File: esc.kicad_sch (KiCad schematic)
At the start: 10 parts, among them J1 Conn_01x02, J2 Conn_01x05, J3 Conn_01x03, U1 AP63205WU

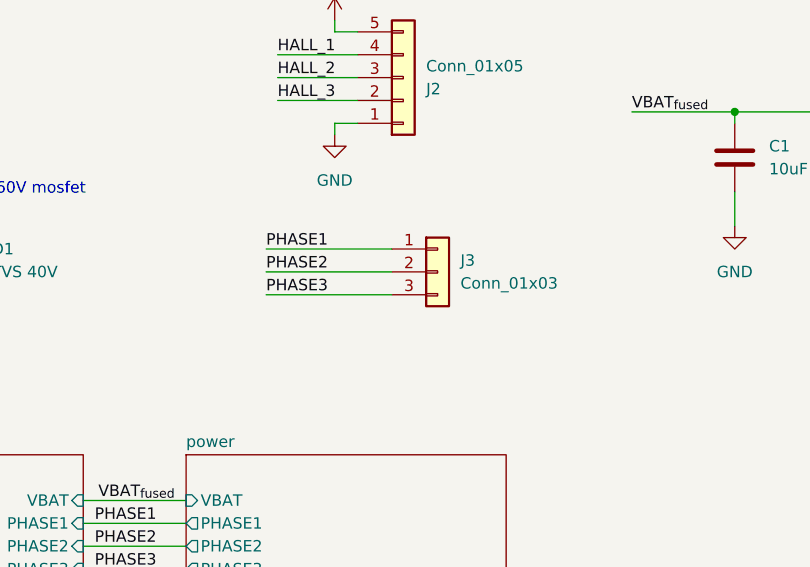
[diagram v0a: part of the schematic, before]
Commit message: added wire step
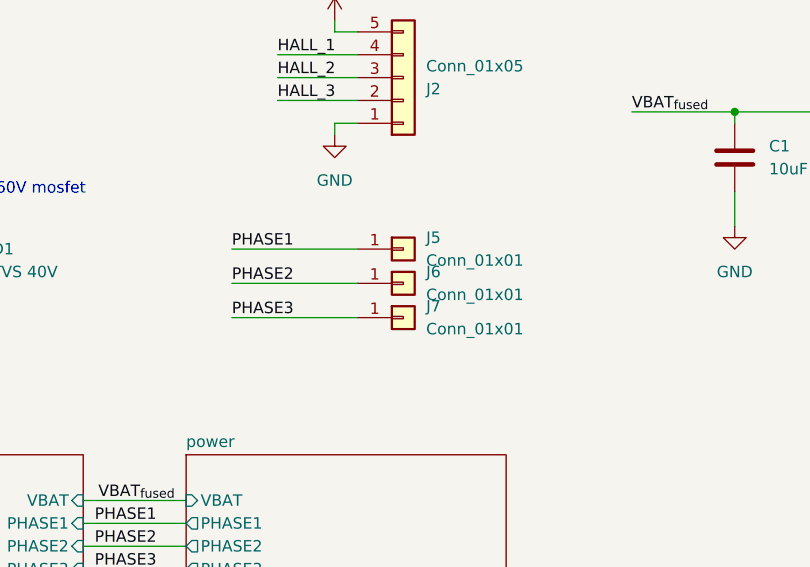
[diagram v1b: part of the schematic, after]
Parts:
- removed J3: Conn_01x03, symbol Connector_Generic:Conn_01x03
- added J5, J6, J7: Conn_01x01, MountingHole:MountingHole_3mm_Pad_Via, symbol Connector_Generic:Conn_01x01
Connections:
- net PHASE1: now also J5.1 (Pin_1)
- net PHASE2: now also J6.1 (Pin_1)
- net PHASE3: now also J7.1 (Pin_1)
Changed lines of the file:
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@@
 	(wire
 		(pts
-			(xy 222.25 96.52) (xy 236.22 96.52)
+			(xy 218.44 96.52) (xy 232.41 96.52)
 		)
 		(stroke
@@
 	(wire
 		(pts
-			(xy 222.25 101.6) (xy 236.22 101.6)
+			(xy 218.44 104.14) (xy 232.41 104.14)
 		)
 		(stroke
@@
 	(wire
 		(pts
-			(xy 222.25 99.06) (xy 236.22 99.06)
+			(xy 218.44 100.33) (xy 232.41 100.33)
 		)
 		(stroke
@@
 	)
 	(label "PHASE2"
-		(at 222.25 99.06 0)
+		(at 218.44 100.33 0)
 		(effects
 			(font
@@
 	)
 	(label "PHASE3"
-		(at 222.25 101.6 0)
+		(at 218.44 104.14 0)
 		(effects
 			(font
@@
 	)
 	(label "PHASE1"
-		(at 222.25 96.52 0)
+		(at 218.44 96.52 0)
 		(effects
 			(font
@@
 	)
 	(symbol
+		(lib_id "Connector_Generic:Conn_01x01")
+		(at 237.49 104.14 0)
+		(unit 1)
+		(body_style 1)
+		(exclude_from_sim no)
+		(in_bom yes)
+		(on_board yes)
+		(in_pos_files yes)
+		(dnp no)
+		(fields_autoplaced yes)
+		(property "Reference" "J7"
+			(at 240.03 102.8699 0)
+			(show_name no)
+			(do_not_autoplace no)
+			(effects
+				(font
+					(size 1.27 1.27)
+				)
+				(justify left)
+			)
+		)
+		(property "Value" "Conn_01x01"
+			(at 240.03 105.4099 0)
+			(show_name no)
+			(do_not_autoplace no)
+			(effects
+				(font
+					(size 1.27 1.27)
+				)
+				(justify left)
+			)
+		)
+		(property "Footprint" "MountingHole:MountingHole_3mm_Pad_Via"
+			(at 237.49 104.14 0)
+			(hide yes)
+			(show_name no)
+			(do_not_autoplace no)
+			(effects
+				(font
+					(size 1.27 1.27)
+				)
+			)
+		)
+		(property "Datasheet" ""
+			(at 237.49 104.14 0)
+			(hide yes)
+			(show_name no)
+			(do_not_autoplace no)
+			(effects
+				(font
+					(size 1.27 1.27)
+				)
+			)
+		)
+		(property "Description" "Generic connector, single row, 01x01, script generated (kicad-library-utils/schlib/autogen/connector/)"
+			(at 237.49 104.14 0)
+			(hide yes)
+			(show_name no)
+			(do_not_autoplace no)
+			(effects
+				(font
+					(size 1.27 1.27)
+				)
+			)
+		)
+		(pin "1"
+		)
+		(instances
+			(project "esc"
+				(path "/3007d2b9-1a69-4117-bc7c-a9e99ed2a97d"
+					(reference "J7")
+					(unit 1)
+				)
+			)
+		)
+	)
+	(symbol
+		(lib_id "Connector_Generic:Conn_01x01")
+		(at 237.49 100.33 0)
+		(unit 1)
+		(body_style 1)
+		(exclude_from_sim no)
+		(in_bom yes)
+		(on_board yes)
+		(in_pos_files yes)
+		(dnp no)
+		(fields_autoplaced yes)
+		(property "Reference" "J6"
+			(at 240.03 99.0599 0)
+			(show_name no)
+			(do_not_autoplace no)
+			(effects
+				(font
+					(size 1.27 1.27)
+				)
+				(justify left)
+			)
+		)
+		(property "Value" "Conn_01x01"
+			(at 240.03 101.5999 0)
+			(show_name no)
+			(do_not_autoplace no)
+			(effects
+				(font
+					(size 1.27 1.27)
+				)
+				(justify left)
+			)
+		)
+		(property "Footprint" "MountingHole:MountingHole_3mm_Pad_Via"
+			(at 237.49 100.33 0)
+			(hide yes)
+			(show_name no)
+			(do_not_autoplace no)
+			(effects
+				(font
+					(size 1.27 1.27)
+				)
+			)
+		)
+		(property "Datasheet" ""
+			(at 237.49 100.33 0)
+			(hide yes)
+			(show_name no)
+			(do_not_autoplace no)
+			(effects
+				(font
+					(size 1.27 1.27)
+				)
+			)
+		)
+		(property "Description" "Generic connector, single row, 01x01, script generated (kicad-library-utils/schlib/autogen/connector/)"
+			(at 237.49 100.33 0)
+			(hide yes)
+			(show_name no)
+			(do_not_autoplace no)
+			(effects
+				(font
+					(size 1.27 1.27)
+				)
+			)
+		)
+		(pin "1"
+		)
+		(instances
+			(project "esc"
+				(path "/3007d2b9-1a69-4117-bc7c-a9e99ed2a97d"
+					(reference "J6")
+					(unit 1)
+				)
+			)
+		)
+	)
+	(symbol
 		(lib_id "Device:C")
 		(at 318.77 83.82 90)
@@
 	)
 	(symbol
-		(lib_id "Connector_Generic:Conn_01x03")
-		(at 241.3 99.06 0)
+		(lib_id "Connector_Generic:Conn_01x01")
+		(at 237.49 96.52 0)
 		(unit 1)
 		(body_style 1)
@@
 		(dnp no)
 		(fields_autoplaced yes)
-		(property "Reference" "J3"
-			(at 243.84 97.7899 0)
+		(property "Reference" "J5"
+			(at 240.03 95.2499 0)
 			(show_name no)
 			(do_not_autoplace no)
@@
 			)
 		)
-		(property "Value" "Conn_01x03"
-			(at 243.84 100.3299 0)
+		(property "Value" "Conn_01x01"
+			(at 240.03 97.7899 0)
 			(show_name no)
 			(do_not_autoplace no)
@@
 			)
 		)
-		(property "Footprint" ""
-			(at 241.3 99.06 0)
+		(property "Footprint" "MountingHole:MountingHole_3mm_Pad_Via"
+			(at 237.49 96.52 0)
 			(hide yes)
 			(show_name no)
@@
 		)
 		(property "Datasheet" ""
-			(at 241.3 99.06 0)
-			(hide yes)
-			(show_name no)
-			(do_not_autoplace no)
-			(effects
-				(font
-					(size 1.27 1.27)
-				)
-			)
-		)
-		(property "Description" "Generic connector, single row, 01x03, script generated (kicad-library-utils/schlib/autogen/connector/)"
-			(at 241.3 99.06 0)
-			(hide yes)
-			(show_name no)
-			(do_not_autoplace no)
-			(effects
-				(font
-					(size 1.27 1.27)
-				)
-			)
-		)
-		(property "Sim.Device" ""
-			(at 241.3 99.06 0)
-			(hide yes)
-			(show_name no)
-			(do_not_autoplace no)
-			(effects
-				(font
-					(size 1.27 1.27)
-				)
-			)
-		)
-		(property "Sim.Type" ""
-			(at 241.3 99.06 0)
-			(hide yes)
-			(show_name no)
-			(do_not_autoplace no)
-			(effects
-				(font
-					(size 1.27 1.27)
-				)
-			)
-		)
-		(pin "3"
-		)
-		(pin "2"
+			(at 237.49 96.52 0)
+			(hide yes)
+			(show_name no)
+			(do_not_autoplace no)
+			(effects
+				(font
+					(size 1.27 1.27)
+				)
+			)
+		)
+		(property "Description" "Generic connector, single row, 01x01, script generated (kicad-library-utils/schlib/autogen/connector/)"
+			(at 237.49 96.52 0)
+			(hide yes)
+			(show_name no)
+			(do_not_autoplace no)
+			(effects
+				(font
+					(size 1.27 1.27)
+				)
+			)
 		)
 		(pin "1"
@@
 			(project "esc"
 				(path "/3007d2b9-1a69-4117-bc7c-a9e99ed2a97d"
-					(reference "J3")
+					(reference "J5")
 					(unit 1)
 				)
